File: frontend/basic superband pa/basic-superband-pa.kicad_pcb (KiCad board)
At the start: 2 copper layers, 64.4 x 78.6 mm, 69 parts, among them CN1 EDGE, CN2 BREAKOUT, K1 D3002, K2 D3002, P1 BNC, P2 CONN_02X01, P3 CONN_01X02, Q1 NPN, Q2 PNP, Q3 RD16HHF1, Q4 NPN, T1 TRANSFO, T2 8:1, T3 4:1, T4 OUT_TRANSF, U1 LP2951-50D

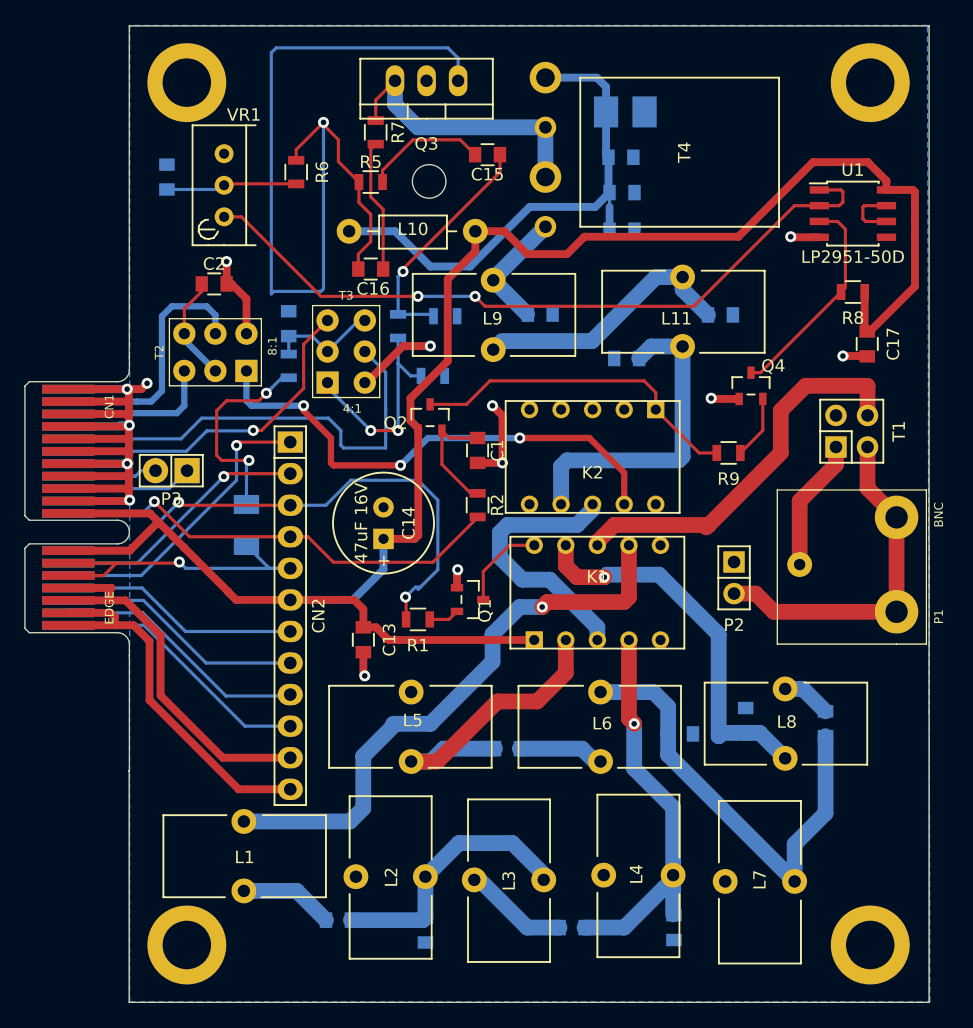
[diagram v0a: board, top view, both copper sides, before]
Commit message: Upload latest pcb changes
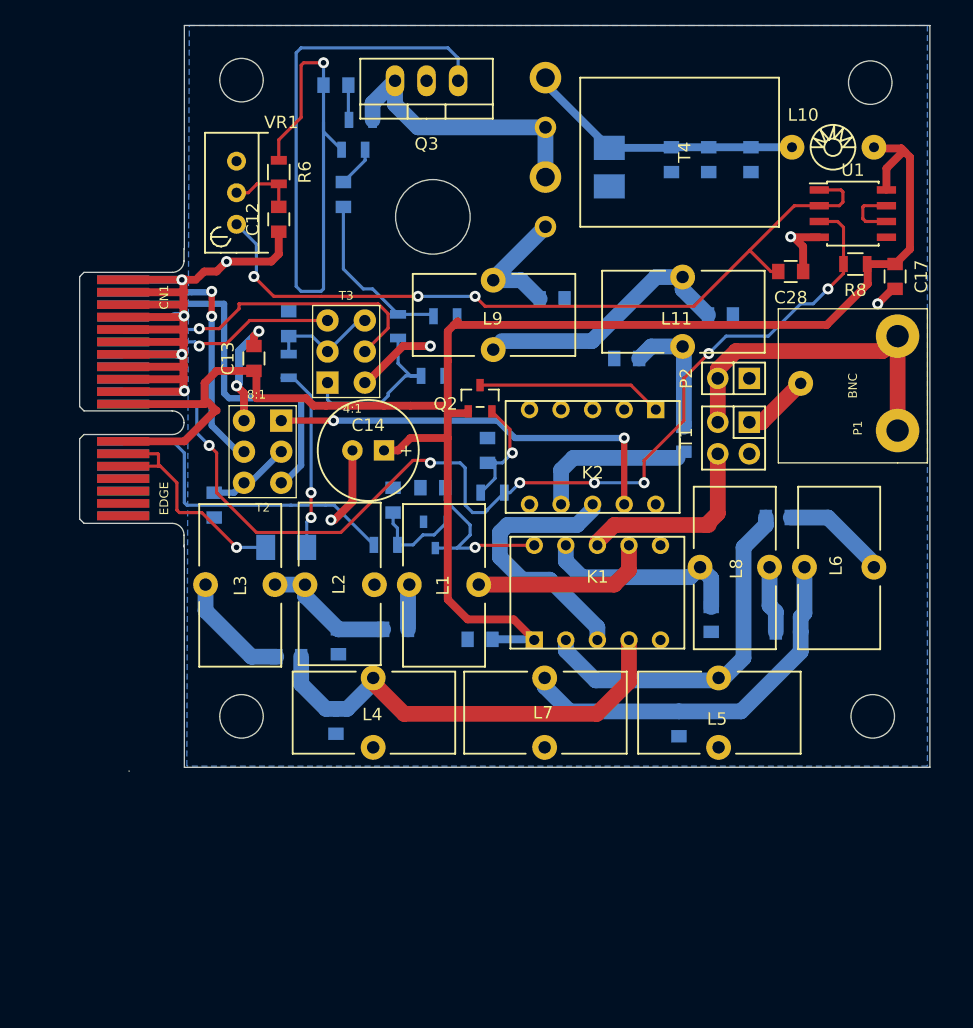
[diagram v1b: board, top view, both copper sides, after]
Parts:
- removed CN2: BREAKOUT, Pin_Headers:Pin_Header_Straight_1x12
- removed MH (x4): VAL**, HERMESLITE:MH
- removed MountingHole_2-7mm: VAL**, Mounting_Holes:MountingHole_2-7mm
- removed P3: CONN_01X02, Pin_Headers:Pin_Header_Straight_1x02
- removed Q4: NPN, Transistors_SMD:sot23
- removed R9: 4.99k, HERMESLITE:R_0805
- added C25: 0.01uF, HERMESLITE:C_0805, B.Cu at (151.2, 73.2)
- added C26: 0.01uF, HERMESLITE:C_0805, B.Cu at (158.2, 84.4)
- added C27: 0.01uF, HERMESLITE:C_0805, B.Cu at (154.4, 72.2)
- added C28: 0.01uF, HERMESLITE:C_0805, F.Cu at (183.2, 54.8)
- added C29: 0.1uF, HERMESLITE:C_0805, B.Cu at (174.6, 68.3)
- added MountingHole_3-5mm: VAL**, Mounting_Holes:MountingHole_3-5mm, F.Cu at (189.8, 90.6)
- added MountingHole_3-5mm: VAL**, Mounting_Holes:MountingHole_3-5mm, F.Cu at (139.0, 90.6)
- added MountingHole_3-5mm: VAL**, Mounting_Holes:MountingHole_3-5mm, F.Cu at (189.6, 39.6)
- added MountingHole_3-5mm: VAL**, Mounting_Holes:MountingHole_3-5mm, F.Cu at (139.0, 39.4)
- added MountingHole_6mm: VAL**, Mounting_Holes:MountingHole_6mm, F.Cu at (154.4, 50.4)
- C1, C15, C16, C2, Q1, R1, R2, R5, R7: moved to B.Cu
- C12: moved to F.Cu
- L10: footprint Choke_Axial_ThroughHole:Choke_Horizontal_RM10mm -> Choke_Toroid_ThroughHole:Choke_Toroid_horizontal_Diameter3-5mm_Amidon-T12
- moved L5 38.7 mm to (184.0, 87.0), turned to 180 degrees
- moved L2 38.2 mm to (143.6, 73.4), turned to 270 degrees
- moved L10 34.5 mm to (186.6, 44.8)
- moved L3 32.1 mm to (142.2, 86.6)
- moved C7 31.9 mm to (146.6, 91.0)
- moved C6 31.5 mm to (142.8, 85.8)
- moved L6 30.6 mm to (190.4, 85.2), turned to 90 degrees
- moved L4 29.2 mm to (156.2, 87.0), turned to 180 degrees
- moved C8 28.7 mm to (182.2, 74.6)
- moved L7 27.4 mm to (170.0, 87.0), turned to 180 degrees
- moved C13 24.3 mm to (140.0, 61.8), turned to 90 degrees
- moved C5 24.2 mm to (146.8, 84.6)
- moved C4 23.8 mm to (151.4, 83.6), turned to 180 degrees
- moved C2 17.8 mm to (136.8, 73.6), turned to 270 degrees
- moved L1 17.5 mm to (158.6, 86.6), turned to 90 degrees
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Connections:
- CN1 pad A16: Net-(CN1-PadA15) -> Net-(CN1-PadA16)
- CN1 pad A18: Net-(CN1-PadA17) -> Net-(CN1-PadA18)
- K2 pad 7: Net-(C24-Pad2) -> Net-(C29-Pad1)
- R8 pad 2: Net-(Q4-Pad3) -> PTT#
- U1 pad 3: Net-(Q4-Pad3) -> PTT#
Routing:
- net PTT#: track 36.9 -> 88.3 mm, vias 1 -> 7
- net Net-(K1-Pad7): track 46.6 -> 14.6 mm, vias 1 -> 0
- net Net-(CN1-PadA17): track 30.6 -> 0.00 mm
- net Net-(CN1-PadA15): track 30.4 -> 0.00 mm
- net Net-(CN1-PadB14): track 23.9 -> 0.00 mm, vias 1 -> 0
- net Net-(CN1-PadB18): track 21.2 -> 0.00 mm
- net Net-(CN1-PadB13): track 20.8 -> 0.00 mm, vias 1 -> 0
- net Net-(CN1-PadB17): track 20.7 -> 0.00 mm
- net Net-(CN1-PadB16): track 19.9 -> 0.00 mm
- net Net-(CN1-PadB15): track 19.3 -> 0.00 mm
- net Net-(C19-Pad2): track 41.4 -> 23.1 mm
- net GPIO0: track 44.1 -> 26.0 mm, vias 2 -> 0
- net Net-(Q4-Pad3): track 17.5 -> 0.00 mm
- net Net-(CN1-PadB3): track 12.4 -> 29.4 mm
- net Net-(K1-Pad8): track 31.9 -> 15.9 mm
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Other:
- board size 64.4 x 78.6 mm -> 64.5 x 60 mm
